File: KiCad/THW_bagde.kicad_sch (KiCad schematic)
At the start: 37 parts, among them J1 USB_B, J2 Conn_02x03_Odd_Even, SW1 SW_Push, SW2 SW_Push, SW3 SW_Push, U1 ATmega328-P, Y1 Crystal

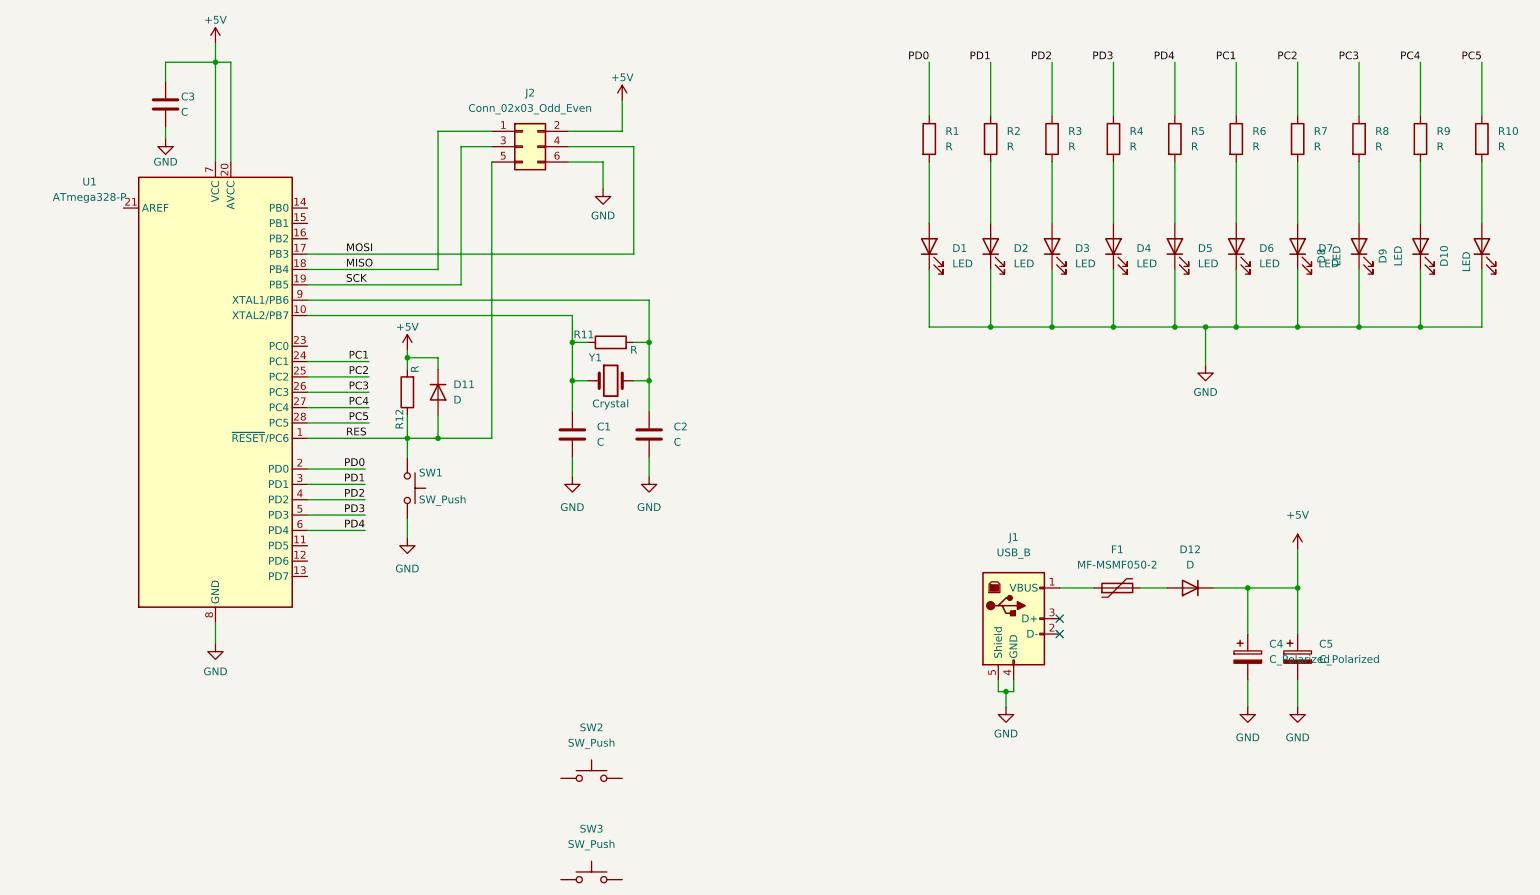
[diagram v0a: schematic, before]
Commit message: adding firmware for tests
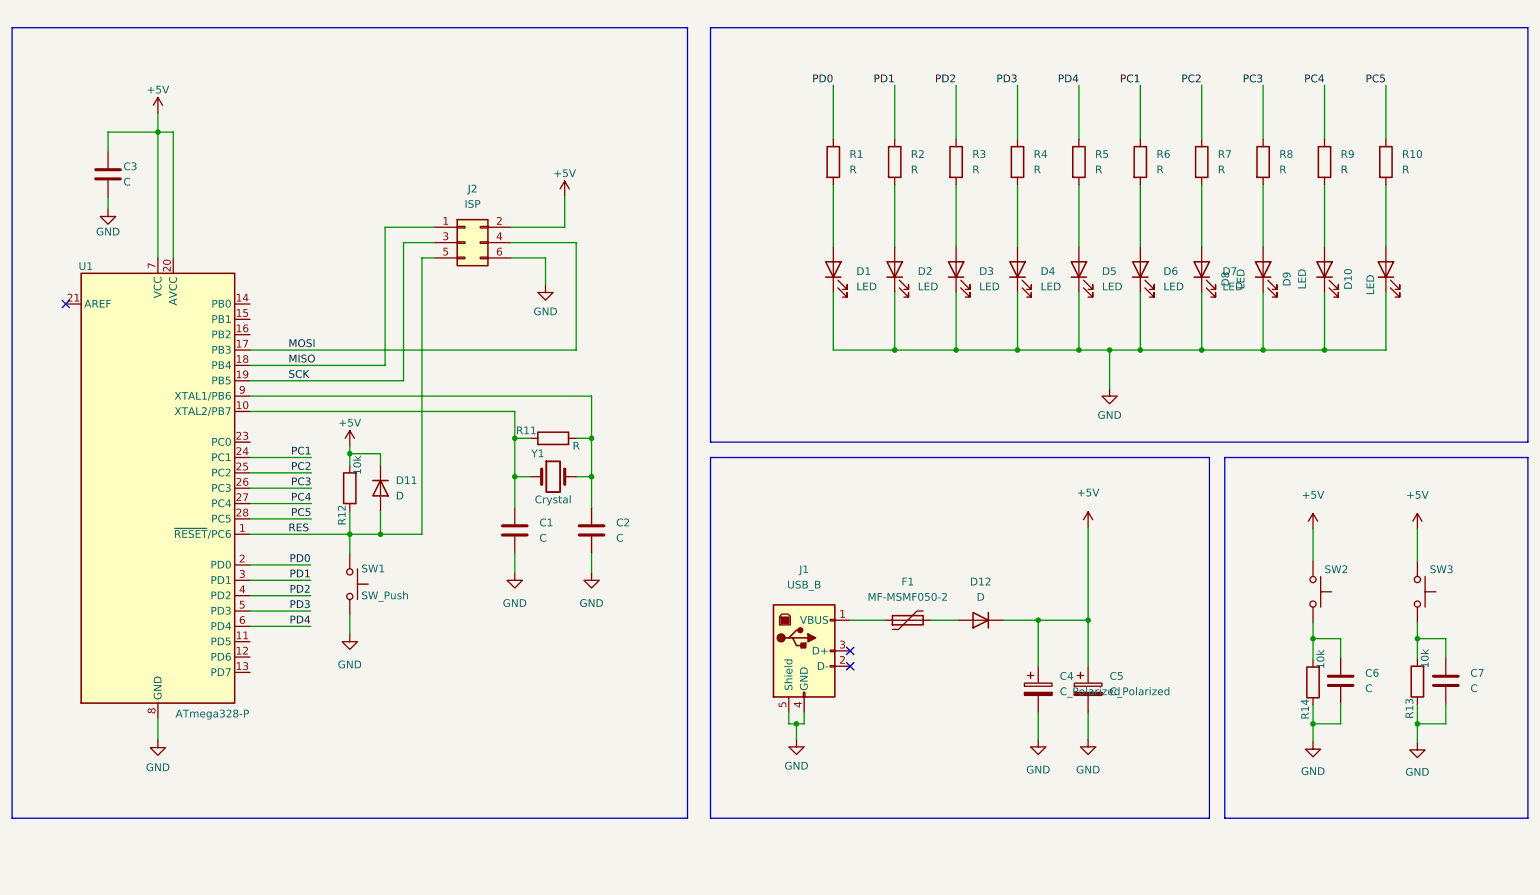
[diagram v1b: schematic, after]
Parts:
- added C6, C7: C, Capacitor_THT:C_Disc_D3.8mm_W2.6mm_P2.50mm, symbol Device:C
- added R13, R14: 10k, Resistor_THT:R_Axial_DIN0207_L6.3mm_D2.5mm_P10.16mm_Horizontal, symbol Device:R
- J2: value Conn_02x03_Odd_Even -> ISP
- R12: value R -> 10k
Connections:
- net +5V: now also SW2.1, SW3.1
- net GND: now also C6.2, C7.2, R13.1, R14.1
- net at SW2.2: now also C6.1, R14.2
- net at SW3.2: now also C7.1, R13.2
- no-connect marks 2 -> 3
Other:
- moved on the sheet: C1, C2, C3, C4, C5, D1, D10, D11, D12, D2, D3, D4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
